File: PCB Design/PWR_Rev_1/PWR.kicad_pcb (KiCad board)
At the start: 2 copper layers, 40 x 65 mm, 61 parts, among them J1 Conn_01x24_Pin, J2 Conn_01x24_Pin, U1 LMR33630ADDA, U2 LMR33630ADDA, U3 TPS55340RTER

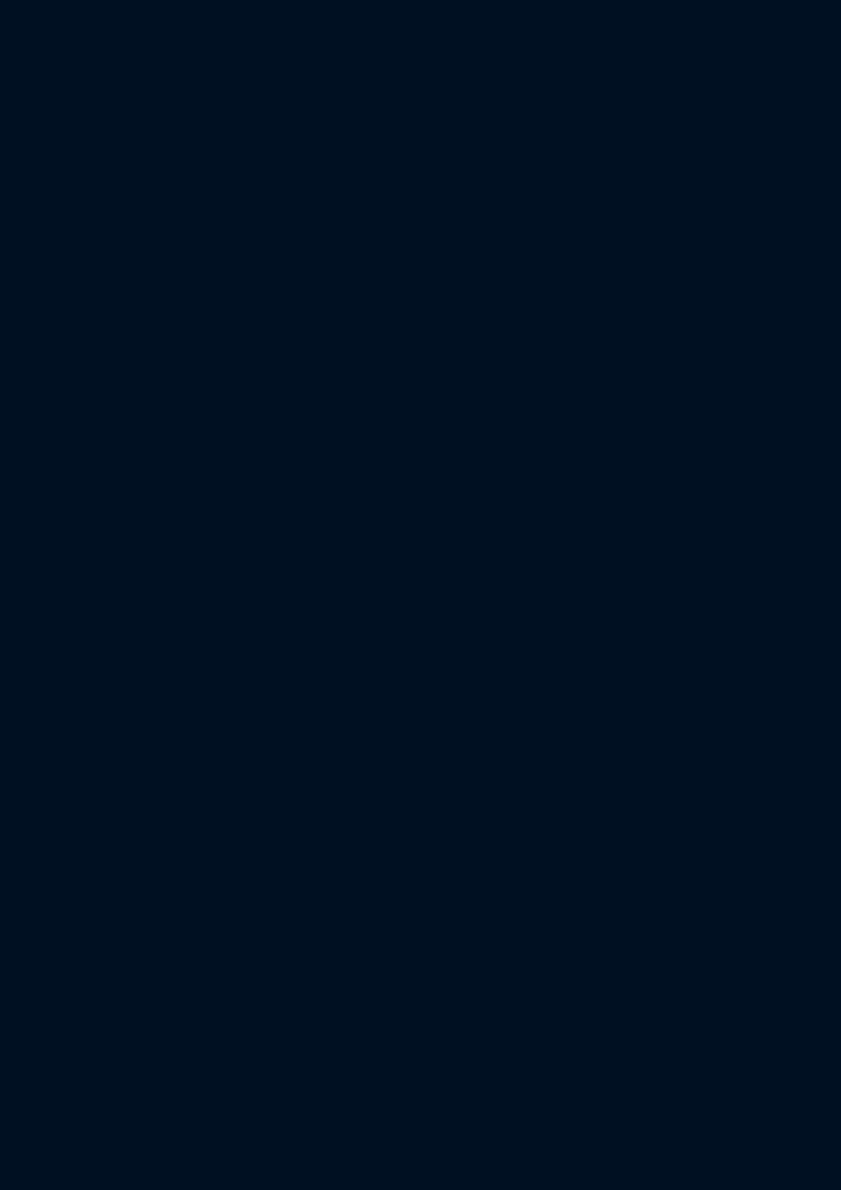
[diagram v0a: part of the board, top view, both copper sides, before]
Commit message: Updated
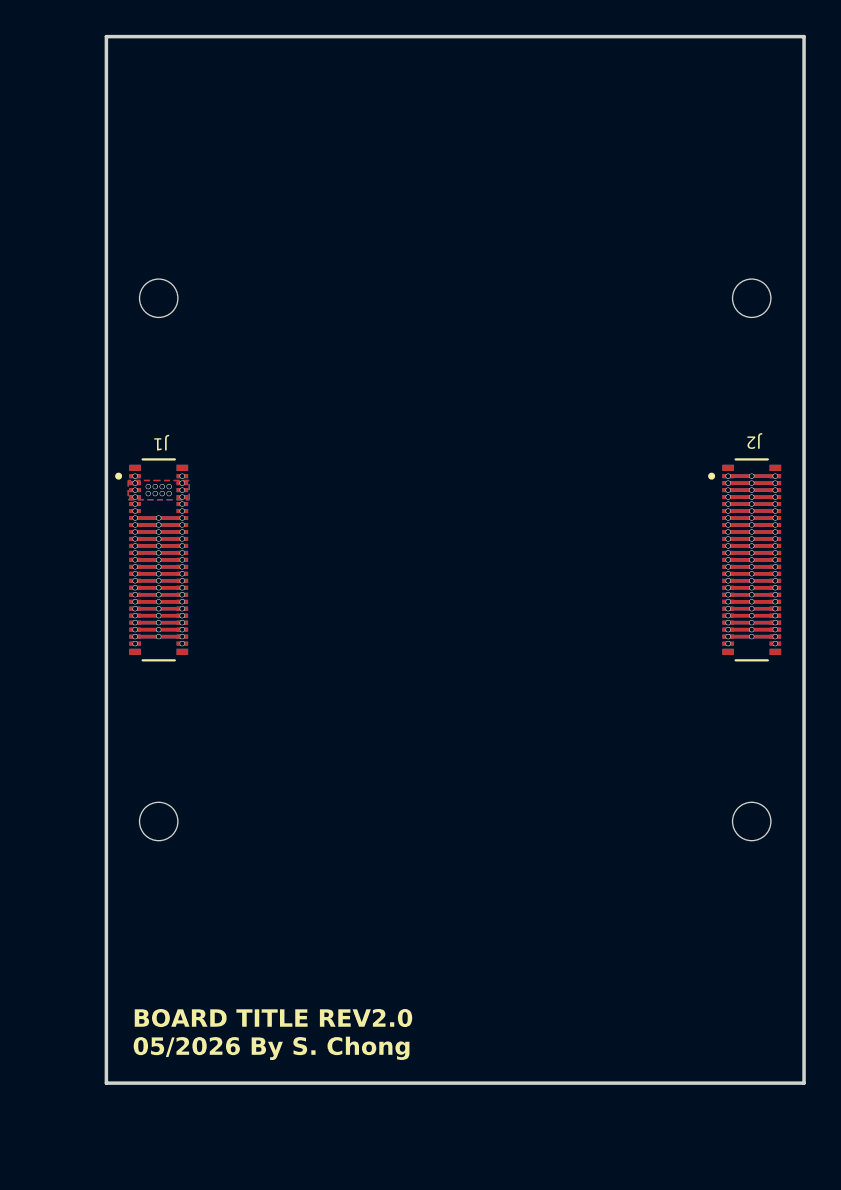
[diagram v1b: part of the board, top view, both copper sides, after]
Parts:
- added J1: Conn_02x25_Odd_Even, CONTROL:HIROSE_DF40C-50DP-0.4V_51_, F.Cu at (208.7, 73.0)
- added J2: Conn_02x25_Odd_Even, CONTROL:HIROSE_DF40C-50DP-0.4V_51_, F.Cu at (242.7, 73.0)
- added J3: Conn_02x25_Odd_Even, CONTROL:HIROSE_DF40C-50DP-0.4V_51_, B.Cu at (208.7, 73.0)
- added J4: Conn_02x25_Odd_Even, CONTROL:HIROSE_DF40C-50DP-0.4V_51_, B.Cu at (242.7, 73.0)
- added REF**: MountingHole_2.2mm_M2, MountingHole:MountingHole_2.2mm_M2, F.Cu at (242.7, 58.0)
- added REF**: MountingHole_2.2mm_M2, MountingHole:MountingHole_2.2mm_M2, F.Cu at (242.7, 88.0)
- added REF**: MountingHole_2.2mm_M2, MountingHole:MountingHole_2.2mm_M2, F.Cu at (208.7, 88.0)
- added REF**: MountingHole_2.2mm_M2, MountingHole:MountingHole_2.2mm_M2, F.Cu at (208.7, 58.0)
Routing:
- net /SDA: track 0.00 -> 5.42 mm, vias 0 -> 3
- net /SCL: track 0.00 -> 5.42 mm, vias 0 -> 3
- net /PC9: track 0.00 -> 5.42 mm, vias 0 -> 3
- net /PC8: track 0.00 -> 5.42 mm, vias 0 -> 3
- net /PC7: track 0.00 -> 5.42 mm, vias 0 -> 3
- net /PC6: track 0.00 -> 5.42 mm, vias 0 -> 3
- net /PC5: track 0.00 -> 5.42 mm, vias 0 -> 3
- net /PC4: track 0.00 -> 5.42 mm, vias 0 -> 3
- net /PC3: track 0.00 -> 5.42 mm, vias 0 -> 3
- net /PC13: track 0.00 -> 5.42 mm, vias 0 -> 3
- net /PC0: track 0.00 -> 5.42 mm, vias 0 -> 3
- net /PB6: track 0.00 -> 5.42 mm, vias 0 -> 3
- net /PB5: track 0.00 -> 5.42 mm, vias 0 -> 3
- net /PB15: track 0.00 -> 5.42 mm, vias 0 -> 3
- net /PB14: track 0.00 -> 5.42 mm, vias 0 -> 3
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- added copper zone on B.Cu, net 3.3V
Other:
- board size 40 x 65 mm -> 111.8 x 90.5 mm
- board text added: "BOARD TITLE REV2.0 05/2026 By S. Chong"

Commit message: Revert "Updated"
This reverts commit 89be44ed720659141c8ee702c54a520a60db740f.
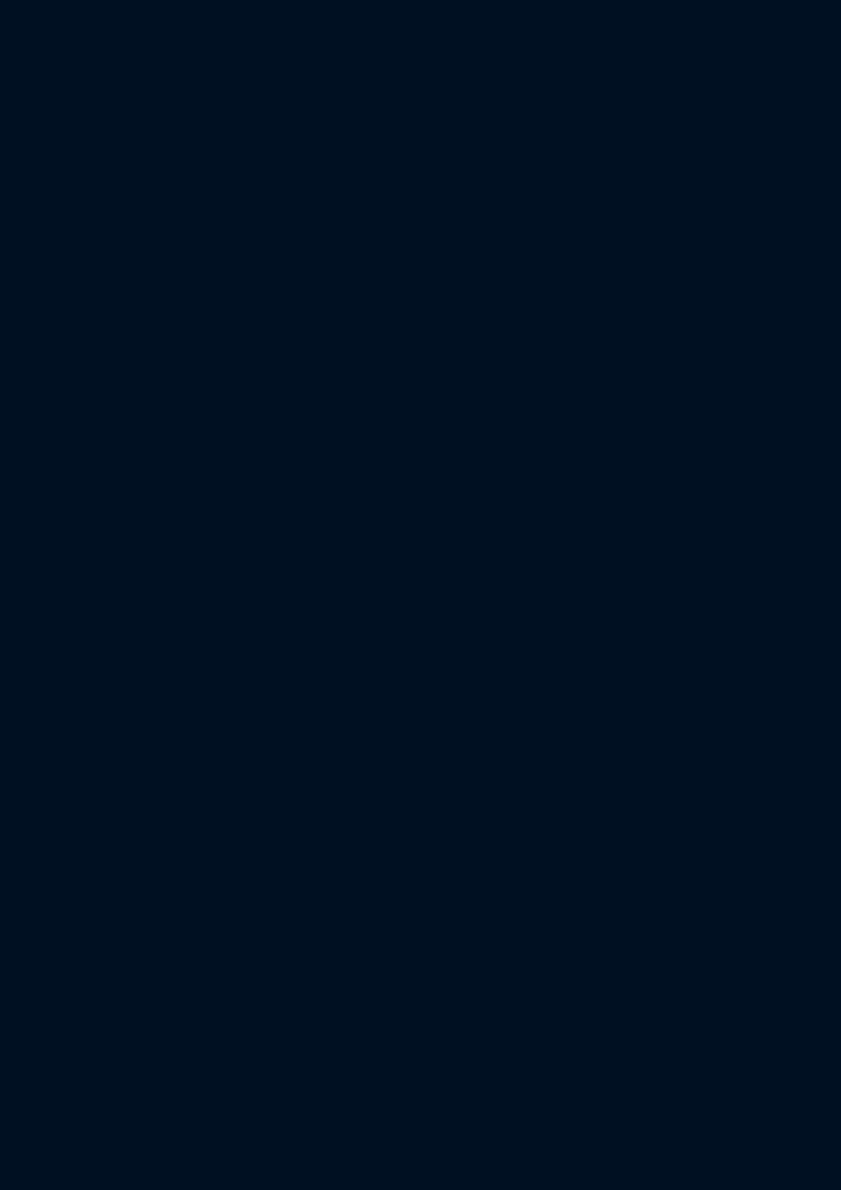
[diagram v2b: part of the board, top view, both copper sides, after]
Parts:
- removed the J1 at (208.7, 73.0)
- removed the J2 at (242.7, 73.0)
- removed J3, J4: Conn_02x25_Odd_Even, CONTROL:HIROSE_DF40C-50DP-0.4V_51_
- removed REF** (x4): MountingHole_2.2mm_M2, MountingHole:MountingHole_2.2mm_M2
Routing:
- net /SDA: track 5.42 -> 0.00 mm, vias 3 -> 0
- net /SCL: track 5.42 -> 0.00 mm, vias 3 -> 0
- net /PC9: track 5.42 -> 0.00 mm, vias 3 -> 0
- net /PC8: track 5.42 -> 0.00 mm, vias 3 -> 0
- net /PC7: track 5.42 -> 0.00 mm, vias 3 -> 0
- net /PC6: track 5.42 -> 0.00 mm, vias 3 -> 0
- net /PC5: track 5.42 -> 0.00 mm, vias 3 -> 0
- net /PC4: track 5.42 -> 0.00 mm, vias 3 -> 0
- net /PC3: track 5.42 -> 0.00 mm, vias 3 -> 0
- net /PC13: track 5.42 -> 0.00 mm, vias 3 -> 0
- net /PC0: track 5.42 -> 0.00 mm, vias 3 -> 0
- net /PB6: track 5.42 -> 0.00 mm, vias 3 -> 0
- net /PB5: track 5.42 -> 0.00 mm, vias 3 -> 0
- net /PB15: track 5.42 -> 0.00 mm, vias 3 -> 0
- net /PB14: track 5.42 -> 0.00 mm, vias 3 -> 0
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- removed copper zone on B.Cu, net 3.3V
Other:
- board size 111.8 x 90.5 mm -> 40 x 65 mm
- board text removed: "BOARD TITLE REV2.0 05/2026 By S. Chong"
